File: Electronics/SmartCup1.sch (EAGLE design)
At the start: 45 parts, among them IC1 REG1117, IC2 REG1117

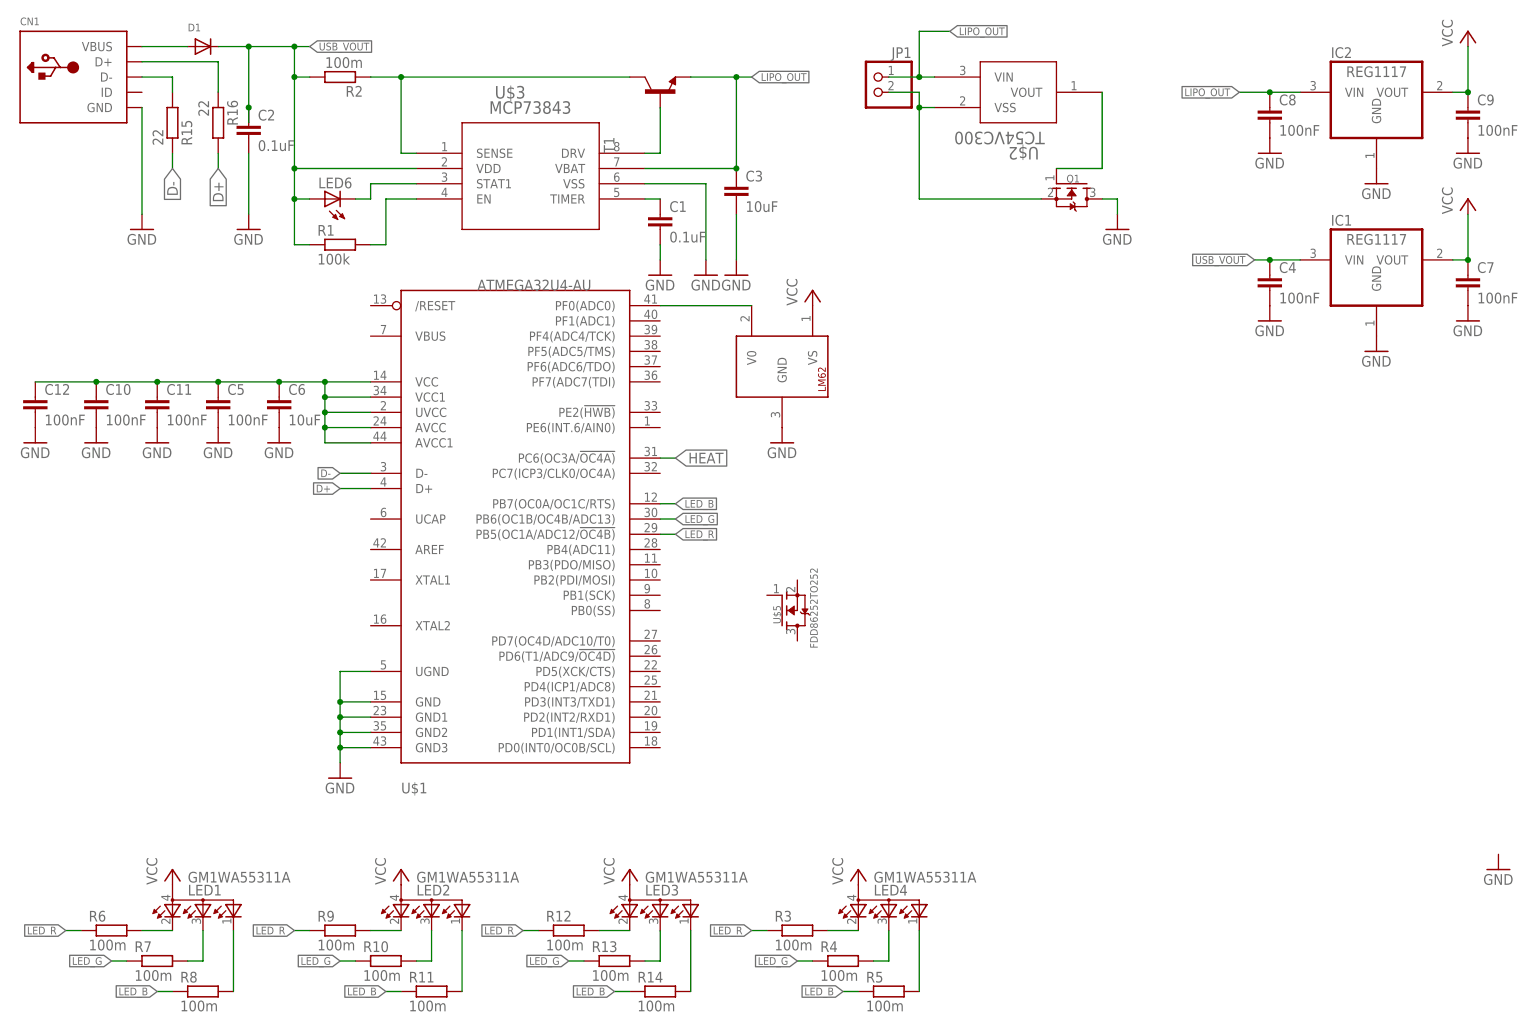
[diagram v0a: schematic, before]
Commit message: Board update
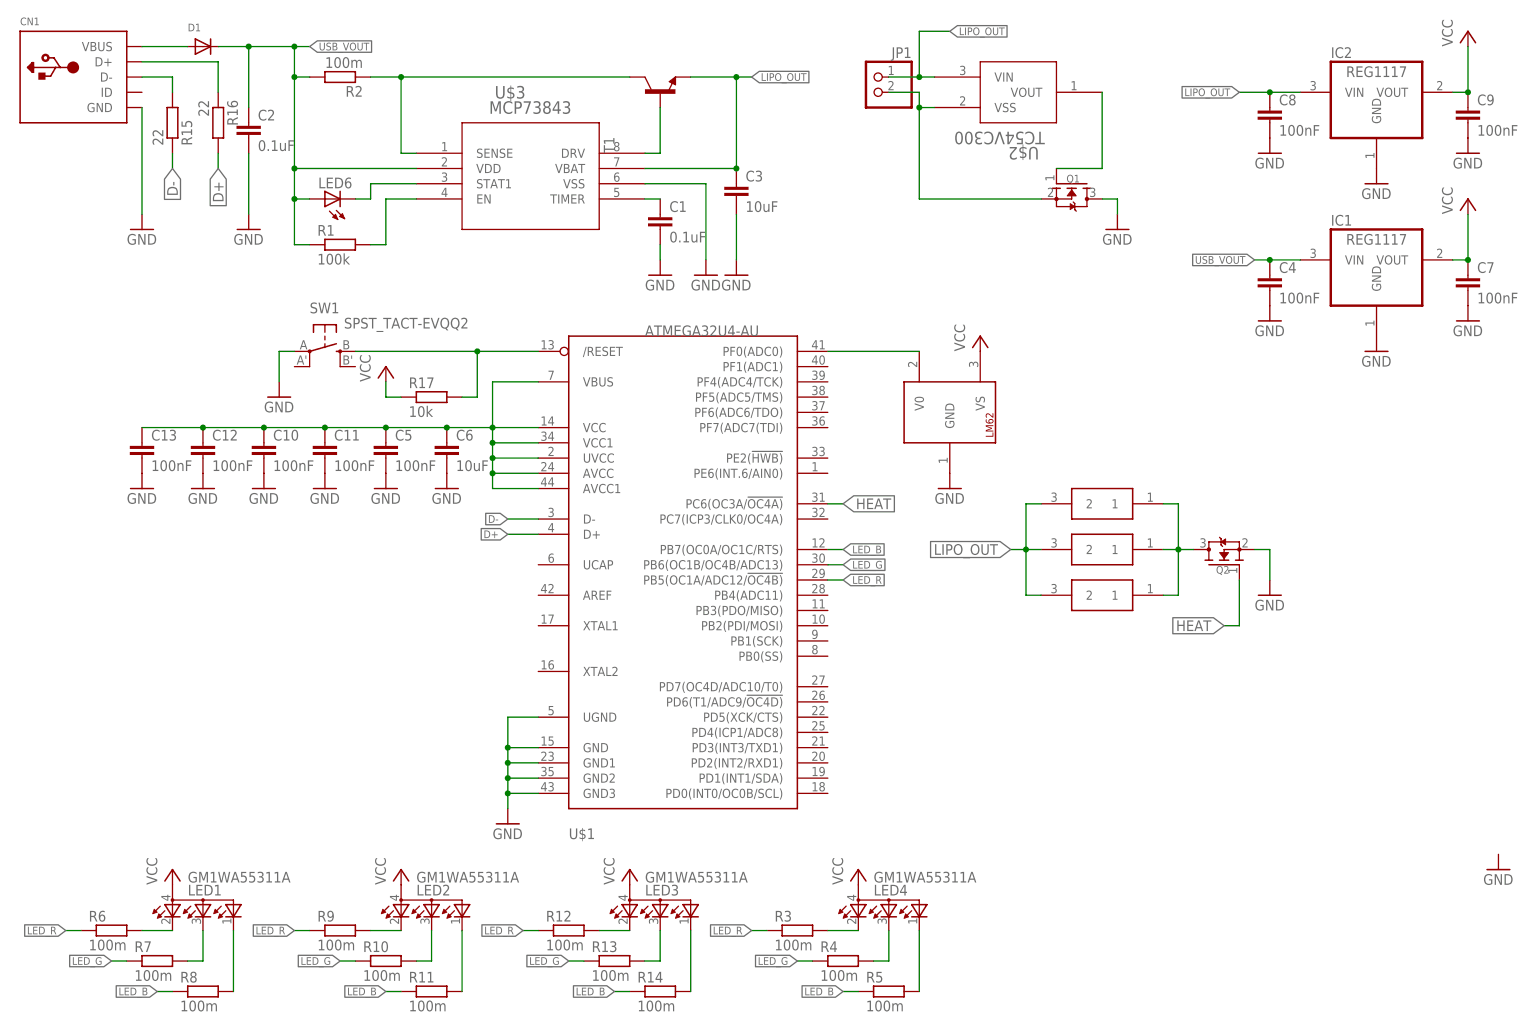
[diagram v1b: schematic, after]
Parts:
- removed U$5: FDD86252TO252, adafruit:FDD86252TO252
- added C13: 100nF, resistor:C-EUC0603
- added Q2: (no value), adafruit:MOSFET-NREFLOW
- added R17: 10k, resistor:R-EU_R0603
- added SW1: SPST_TACT-EVQQ2, adafruit:SPST_TACT-EVQQ2
- added U$6, U$7, U$8: BOURNS_PWR, BOURNS:BOURNS_PWR
- D1: device adafruit:DIODESMA -> adafruit:DIODE_SOD-123FL
- U$4: value LM62 -> LM62TO-92; device LM62:LM62 -> LM62:LM62TO-92
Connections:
- new net N$25: R17.2, SW1.S, U$1./RESET
- new net N$26: Q2.D, U$6.1, U$7.1, U$8.1
- net GND: now also C13.2, Q2.S, SW1.P
- net HEAT: now also Q2.G
- net LIPO_OUT: now also U$6.2, U$7.2, U$8.2
- net N$20: now also C13.1, U$1.VBUS
- net VCC: now also R17.1
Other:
- moved on the sheet: C10, C11, C12, C5, C6, U$1
